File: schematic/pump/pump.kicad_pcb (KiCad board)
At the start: 2 copper layers, 0 parts

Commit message: PCBs started!
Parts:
- added A0: DRV8825_Carrier, Modules:Pololu_Breakout-16_15.2x20.3mm, F.Cu at (110.0, 40.0)
- added A1: DRV8825_Carrier, Modules:Pololu_Breakout-16_15.2x20.3mm, F.Cu at (110.0, 61.0)
- added A2: DRV8825_Carrier, Modules:Pololu_Breakout-16_15.2x20.3mm, F.Cu at (110.0, 82.0)
- added A3: DRV8825_Carrier, Modules:Pololu_Breakout-16_15.2x20.3mm, F.Cu at (110.0, 103.0)
- added A4: DRV8825_Carrier, Modules:Pololu_Breakout-16_15.2x20.3mm, F.Cu at (110.0, 124.0)
- added A5: DRV8825_Carrier, Modules:Pololu_Breakout-16_15.2x20.3mm, F.Cu at (110.0, 145.0)
- added A6: DRV8825_Carrier, Modules:Pololu_Breakout-16_15.2x20.3mm, F.Cu at (110.0, 166.0)
- added A7: DRV8825_Carrier, Modules:Pololu_Breakout-16_15.2x20.3mm, F.Cu at (110.0, 187.0)
- added C0: 100u, Capacitors_THT:CP_Radial_D6.3mm_P2.50mm, F.Cu at (118.0, 40.5)
- added C1: 100u, Capacitors_THT:CP_Radial_D6.3mm_P2.50mm, F.Cu at (118.0, 61.5)
- added C2: 100u, Capacitors_THT:CP_Radial_D6.3mm_P2.50mm, F.Cu at (118.0, 82.5)
- added C3: 100u, Capacitors_THT:CP_Radial_D6.3mm_P2.50mm, F.Cu at (118.0, 103.5)
- added C4: 100u, Capacitors_THT:CP_Radial_D6.3mm_P2.50mm, F.Cu at (118.0, 124.5)
- added C5: 100u, Capacitors_THT:CP_Radial_D6.3mm_P2.50mm, F.Cu at (118.0, 145.5)
- added C6: 100u, Capacitors_THT:CP_Radial_D6.3mm_P2.50mm, F.Cu at (118.0, 166.5)
- added C7: 100u, Capacitors_THT:CP_Radial_D6.3mm_P2.50mm, F.Cu at (118.0, 187.5)
- added CON1: Main, Socket_Strips:Socket_Strip_Angled_1x15_Pitch2.54mm, F.Cu at (105.4, 104.5)
- added J0: Motor, Pin_Headers:Pin_Header_Straight_1x04_Pitch2.54mm, F.Cu at (127.0, 45.1)
- added J1: Motor, Pin_Headers:Pin_Header_Straight_1x04_Pitch2.54mm, F.Cu at (127.0, 66.1)
- added J2: Motor, Pin_Headers:Pin_Header_Straight_1x04_Pitch2.54mm, F.Cu at (127.0, 87.1)
- added J3: Motor, Pin_Headers:Pin_Header_Straight_1x04_Pitch2.54mm, F.Cu at (127.0, 108.1)
- added J4: Motor, Pin_Headers:Pin_Header_Straight_1x04_Pitch2.54mm, F.Cu at (127.0, 129.1)
- added J5: Motor, Pin_Headers:Pin_Header_Straight_1x04_Pitch2.54mm, F.Cu at (127.0, 150.1)
- added J6: Motor, Pin_Headers:Pin_Header_Straight_1x04_Pitch2.54mm, F.Cu at (127.0, 171.1)
- added J7: Motor, Pin_Headers:Pin_Header_Straight_1x04_Pitch2.54mm, F.Cu at (127.0, 192.1)
- added M0: M0, Pin_Headers:Pin_Header_Straight_2x01_Pitch2.54mm, F.Cu at (105.8, 84.6)
- added M1: M1, Pin_Headers:Pin_Header_Straight_2x01_Pitch2.54mm, F.Cu at (105.8, 87.2)
- added M2: M2, Pin_Headers:Pin_Header_Straight_2x01_Pitch2.54mm, F.Cu at (105.8, 89.8)
- added REF**: MountingHole_3.2mm_M3, Mounting_Holes:MountingHole_3.2mm_M3, F.Cu at (102.2, 205.5)
- added REF**: MountingHole_3.2mm_M3, Mounting_Holes:MountingHole_3.2mm_M3, F.Cu at (102.2, 38.5)
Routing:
- net /GND: track 0.00 -> 494.5 mm
- net /24V: track 0.00 -> 376.0 mm
- net /3.3V: track 0.00 -> 206.9 mm, vias 0 -> 8
- net /~ENABLE: track 0.00 -> 193.6 mm, vias 0 -> 7
- net /M0: track 0.00 -> 186.7 mm, vias 0 -> 7
- net /M1: track 0.00 -> 180.6 mm, vias 0 -> 7
- net /M2: track 0.00 -> 174.6 mm, vias 0 -> 7
- net /DIR: track 0.00 -> 169.0 mm
- net /P7: track 0.00 -> 69.3 mm
- net /P0: track 0.00 -> 57.1 mm
- net /P6: track 0.00 -> 51.6 mm
- net /P1: track 0.00 -> 38.9 mm
- net /P5: track 0.00 -> 33.4 mm
- net /P2: track 0.00 -> 20.8 mm
- net /P4: track 0.00 -> 15.2 mm
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- added copper zone on B.Cu, net /GND
- added copper zone on F.Cu, net /GND
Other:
- board outline added: 31.2 x 174 mm
- net class 24V Power added: clearance 0.1524, trace_width 1.905, via_dia 0.6858, via_drill 0.3302
- net class Default: trace_width 0.1524 -> 0.2032
- net class Power: trace_width 0.4572 -> 0.508
- board text added: "1"
- board text added: "Barbot Pump Driver v1.0"
- board text added: "Red"

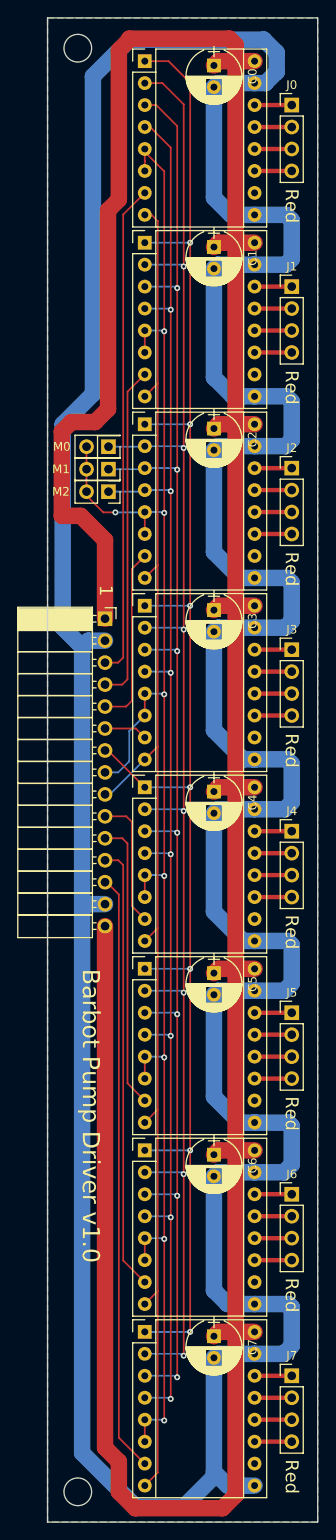
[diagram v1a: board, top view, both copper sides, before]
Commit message: Finished board designs.
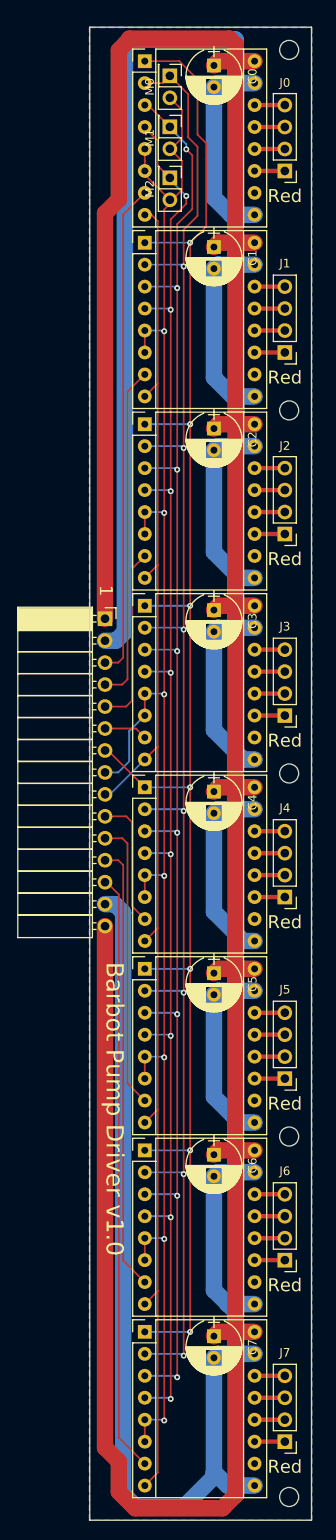
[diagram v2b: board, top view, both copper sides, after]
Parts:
- removed M0: M0, Pin_Headers:Pin_Header_Straight_2x01_Pitch2.54mm
- removed M1: M1, Pin_Headers:Pin_Header_Straight_2x01_Pitch2.54mm
- removed M2: M2, Pin_Headers:Pin_Header_Straight_2x01_Pitch2.54mm
- removed the REF** at (102.2, 205.5)
- removed the REF** at (102.2, 38.5)
- added JP1: M0, Pin_Headers:Pin_Header_Straight_2x01_Pitch2.54mm, F.Cu at (112.9, 41.7)
- added JP2: M1, Pin_Headers:Pin_Header_Straight_2x01_Pitch2.54mm, F.Cu at (112.9, 47.6)
- added JP3: M2, Pin_Headers:Pin_Header_Straight_2x01_Pitch2.54mm, F.Cu at (112.9, 53.5)
- added REF**: MountingHole_2.2mm_M2, Mounting_Holes:MountingHole_2.2mm_M2, F.Cu at (126.6, 164.4)
- added REF**: MountingHole_2.2mm_M2, Mounting_Holes:MountingHole_2.2mm_M2, F.Cu at (126.7, 80.4)
- added REF**: MountingHole_2.2mm_M2, Mounting_Holes:MountingHole_2.2mm_M2, F.Cu at (126.7, 38.7)
- added REF**: MountingHole_2.2mm_M2, Mounting_Holes:MountingHole_2.2mm_M2, F.Cu at (126.7, 206.1)
- added REF**: MountingHole_2.2mm_M2, Mounting_Holes:MountingHole_2.2mm_M2, F.Cu at (126.7, 122.4)
- moved J0 7.66 mm to (126.2, 52.7), turned to 180 degrees
- moved J1 7.66 mm to (126.2, 73.7), turned to 180 degrees
- moved J2 7.66 mm to (126.2, 94.7), turned to 180 degrees
- moved J3 7.66 mm to (126.2, 115.7), turned to 180 degrees
- moved J4 7.66 mm to (126.2, 136.7), turned to 180 degrees
- moved J5 7.66 mm to (126.2, 157.7), turned to 180 degrees
- moved J6 7.66 mm to (126.2, 178.7), turned to 180 degrees
- moved J7 7.66 mm to (126.2, 199.7), turned to 180 degrees
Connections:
- J0 pad 1: /Module0/B2 -> /Module0/A2
- J0 pad 2: /Module0/B1 -> /Module0/A1
- J0 pad 3: /Module0/A1 -> /Module0/B1
- J0 pad 4: /Module0/A2 -> /Module0/B2
- J1 pad 1: /Module1/B2 -> /Module1/A2
- J1 pad 2: /Module1/B1 -> /Module1/A1
- J1 pad 3: /Module1/A1 -> /Module1/B1
- J1 pad 4: /Module1/A2 -> /Module1/B2
- J2 pad 1: /Module2/B2 -> /Module2/A2
- J2 pad 2: /Module2/B1 -> /Module2/A1
- J2 pad 3: /Module2/A1 -> /Module2/B1
- J2 pad 4: /Module2/A2 -> /Module2/B2
- J3 pad 1: /Module3/B2 -> /Module3/A2
- J3 pad 2: /Module3/B1 -> /Module3/A1
- J3 pad 3: /Module3/A1 -> /Module3/B1
- J3 pad 4: /Module3/A2 -> /Module3/B2
- J4 pad 1: /Module4/B2 -> /Module4/A2
- J4 pad 2: /Module4/B1 -> /Module4/A1
- J4 pad 3: /Module4/A1 -> /Module4/B1
- J4 pad 4: /Module4/A2 -> /Module4/B2
- J5 pad 1: /Module5/B2 -> /Module5/A2
- J5 pad 2: /Module5/B1 -> /Module5/A1
- J5 pad 3: /Module5/A1 -> /Module5/B1
- J5 pad 4: /Module5/A2 -> /Module5/B2
- J6 pad 1: /Module6/B2 -> /Module6/A2
- J6 pad 2: /Module6/B1 -> /Module6/A1
- J6 pad 3: /Module6/A1 -> /Module6/B1
- J6 pad 4: /Module6/A2 -> /Module6/B2
- J7 pad 1: /Module7/B2 -> /Module7/A2
- J7 pad 2: /Module7/B1 -> /Module7/A1
- J7 pad 3: /Module7/A1 -> /Module7/B1
- J7 pad 4: /Module7/A2 -> /Module7/B2
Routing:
- net /GND: track 494.5 -> 399.4 mm
- net /24V: track 376.0 -> 368.9 mm
- net /M1: track 180.6 -> 177.4 mm, vias 7 -> 8
- net /M2: track 174.6 -> 172.3 mm, vias 7 -> 8
- net /~ENABLE: track 193.6 -> 195.8 mm
- net /M0: track 186.7 -> 185.5 mm
- net /Module7/B2: track 4.30 -> 3.50 mm
- net /Module7/B1: track 4.30 -> 3.50 mm
- net /Module7/A2: track 4.30 -> 3.50 mm
- net /Module7/A1: track 4.30 -> 3.50 mm
- net /Module6/B2: track 4.30 -> 3.50 mm
- net /Module6/B1: track 4.30 -> 3.50 mm
- net /Module6/A2: track 4.30 -> 3.50 mm
- net /Module6/A1: track 4.30 -> 3.50 mm
- net /Module5/B2: track 4.30 -> 3.50 mm
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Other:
- board size 31.2 x 174 mm -> 25.7 x 172.7 mm

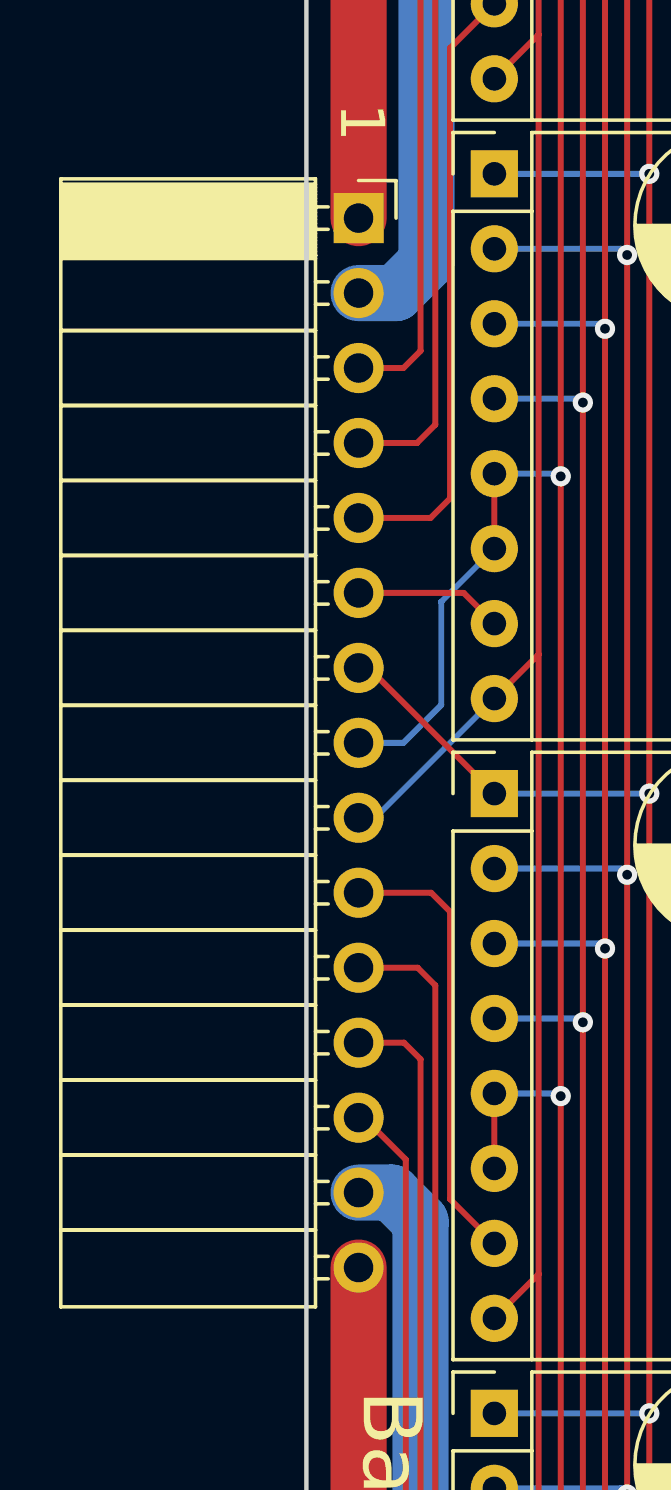
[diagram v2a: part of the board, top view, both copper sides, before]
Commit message: Small tweaks
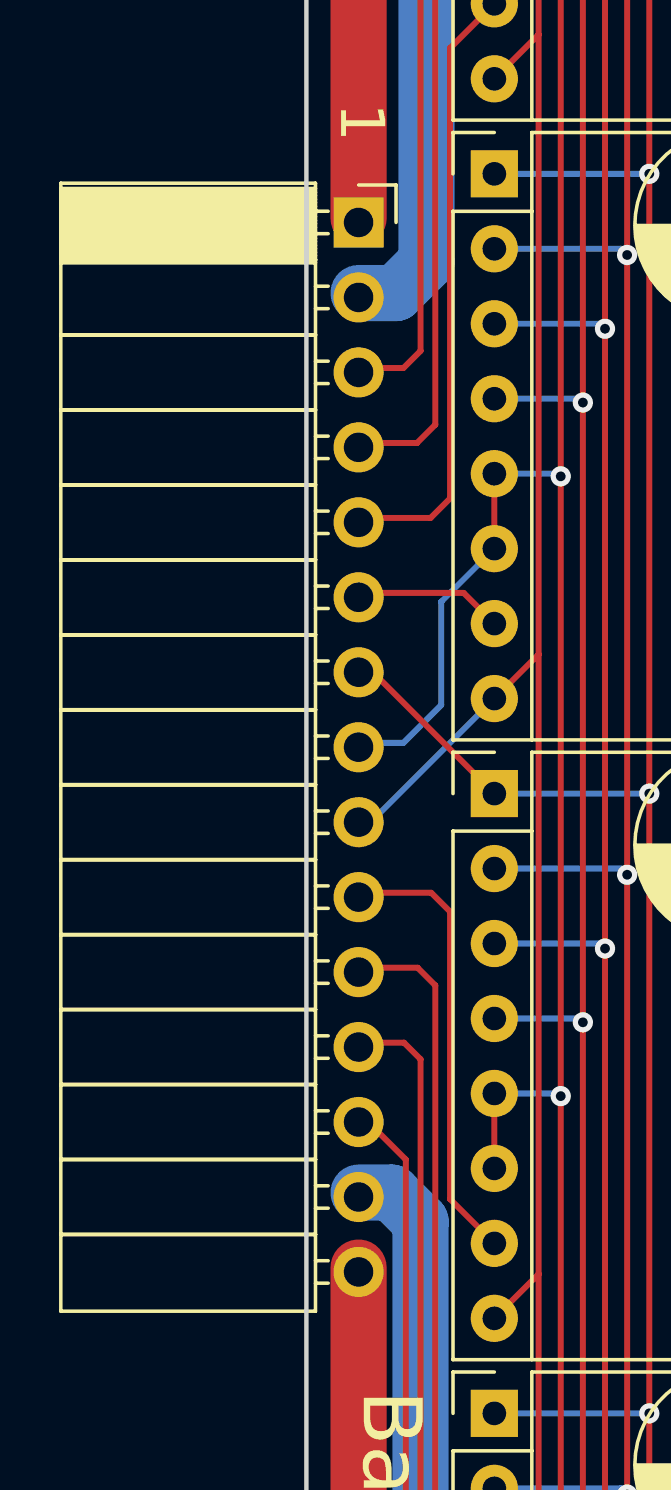
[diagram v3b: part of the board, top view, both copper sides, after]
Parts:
- moved CON1 0.15 mm to (105.4, 104.6)
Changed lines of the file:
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@@
   )
   (module Socket_Strips:Socket_Strip_Angled_1x15_Pitch2.54mm (layer F.Cu)
-    (at 105.4 104.5)
+    (at 105.4 104.648)
     (descr "Through hole angled socket strip, 1x15, 2.54mm pitch, 8.51mm socket length, single row")
     (tags "Through hole angled socket strip THT 1x15 2.54mm single row")
